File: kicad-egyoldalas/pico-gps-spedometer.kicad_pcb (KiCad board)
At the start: 2 copper layers, 88.1 x 75.5 mm, 25 parts, among them J1 Akkumulátor be, J2 TP4056-18650-Charger, J3 uBlox NEO GPS (6M/8M), Q1 PN2222A, U1 RP2040-ZERO, U2 DS18B20, U3 LM7805_TO220, U4 TFT_320x240

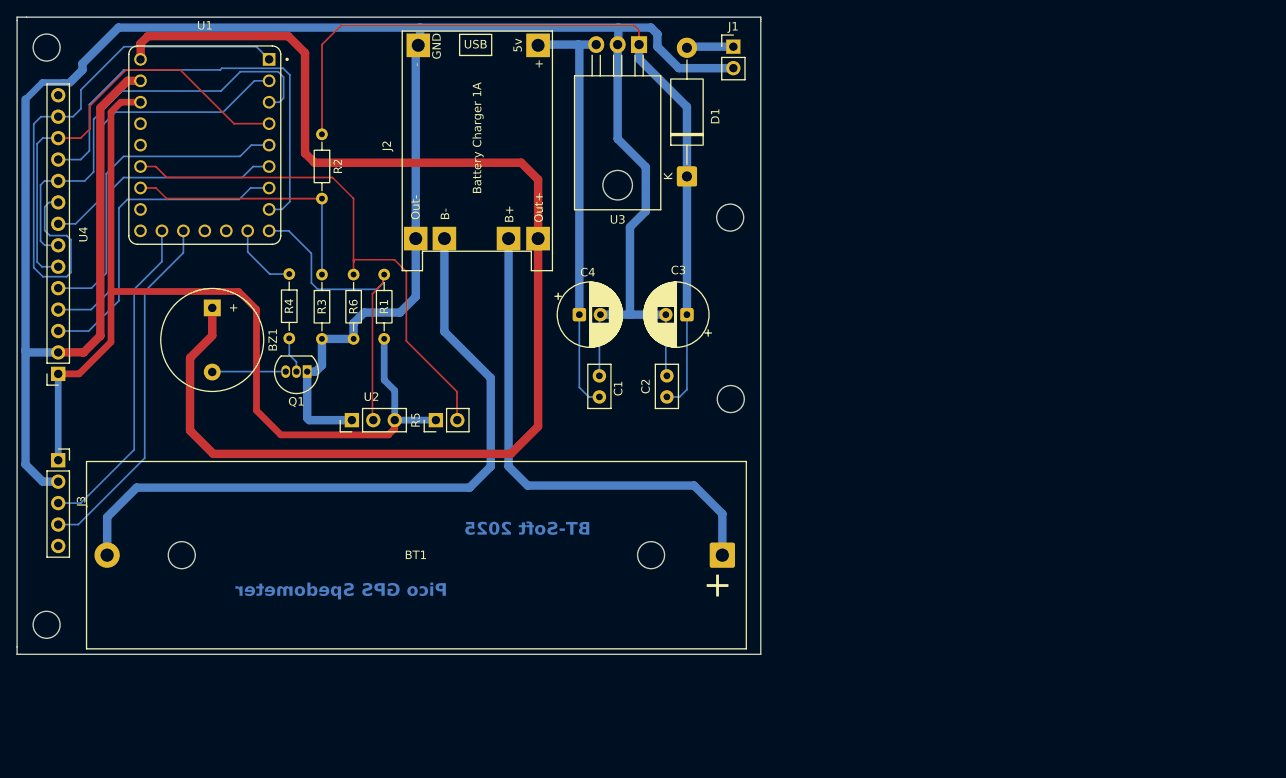
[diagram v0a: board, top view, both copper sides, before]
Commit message: Refactor code structure for improved readability and maintainability
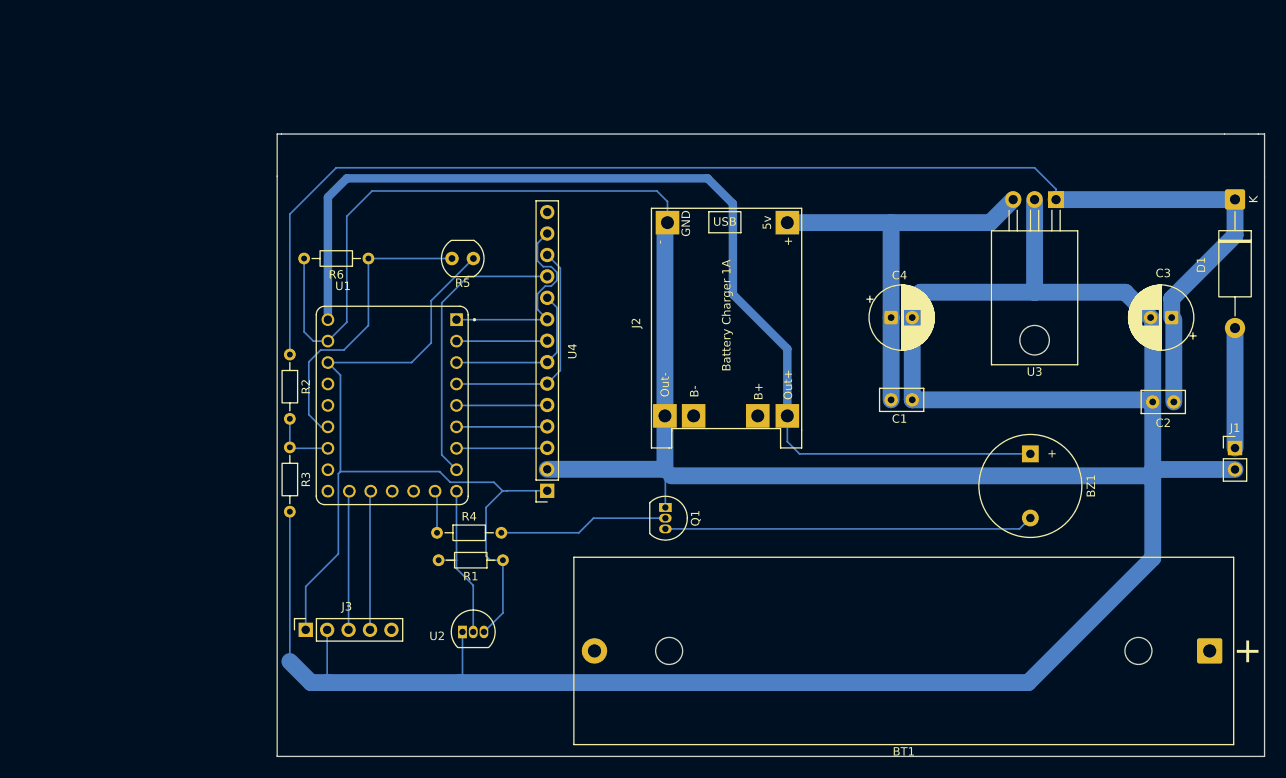
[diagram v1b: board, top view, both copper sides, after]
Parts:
- removed REF** (x4): MountingHole_3.2mm_M3, MountingHole:MountingHole_3.2mm_M3
- R5: footprint Connector_PinHeader_2.54mm:PinHeader_1x02_P2.54mm_Vertical -> OptoDevice:R_LDR_4.9x4.2mm_P2.54mm_Vertical
- U2: footprint Connector_PinHeader_2.54mm:PinHeader_1x03_P2.54mm_Vertical -> Package_TO_SOT_THT:TO-92_Inline
- moved BZ1 98.5 mm to (172.2, 74.4)
- moved J1 76.1 mm to (196.5, 73.7)
- moved D1 65.0 mm to (196.5, 44.2), turned to -90 degrees
- moved C2 60.1 mm to (189.2, 68.2), turned to 180 degrees
- moved U4 59.6 mm to (115.0, 78.8)
- moved BT1 58.9 mm to (193.5, 97.8)
- moved C3 57.4 mm to (189.0, 58.2)
- moved U3 52.7 mm to (175.3, 44.3)
- moved Q1 45.4 mm to (129.0, 80.8), turned to -90 degrees
- moved U1 38.0 mm to (96.6, 68.7)
- moved C4 36.9 mm to (155.8, 58.2)
- moved J2 36.2 mm to (145.2, 45.3)
- moved J3 35.6 mm to (86.4, 95.2), turned to 90 degrees
- moved R4 35.3 mm to (101.9, 83.8), turned to 0 degrees
- moved C1 34.6 mm to (155.8, 68.0), turned to 0 degrees
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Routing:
- net GND: track 303.7 -> 435.4 mm
- net Net-(BT1-2): track 81.7 -> 0.00 mm
- net V-IN-MEAS: track 97.2 -> 160.4 mm
- net Net-(BT1-1): track 59.6 -> 0.00 mm
- net /MISO: track 67.7 -> 24.8 mm
- net Net-(BZ1--): track 8.73 -> 43.8 mm
- net /SCK: track 51.6 -> 19.3 mm
- net /RST: track 38.9 -> 10.8 mm
- net /DC: track 38.9 -> 10.8 mm
- net /CS: track 38.5 -> 10.8 mm
- net +5VBATT: track 152.5 -> 124.9 mm
- net Net-(U1-GP27): track 63.1 -> 35.8 mm
- net /LED: track 37.0 -> 10.8 mm
- net GPS_RXD: track 42.3 -> 16.7 mm
- net /MOSI: track 52.1 -> 27.3 mm
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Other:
- board size 88.1 x 75.5 mm -> 117 x 73.8 mm
- board text removed: "BT-Soft 2025"
- board text removed: "Pico GPS Spedometer"
